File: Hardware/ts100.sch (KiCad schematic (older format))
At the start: 51 parts

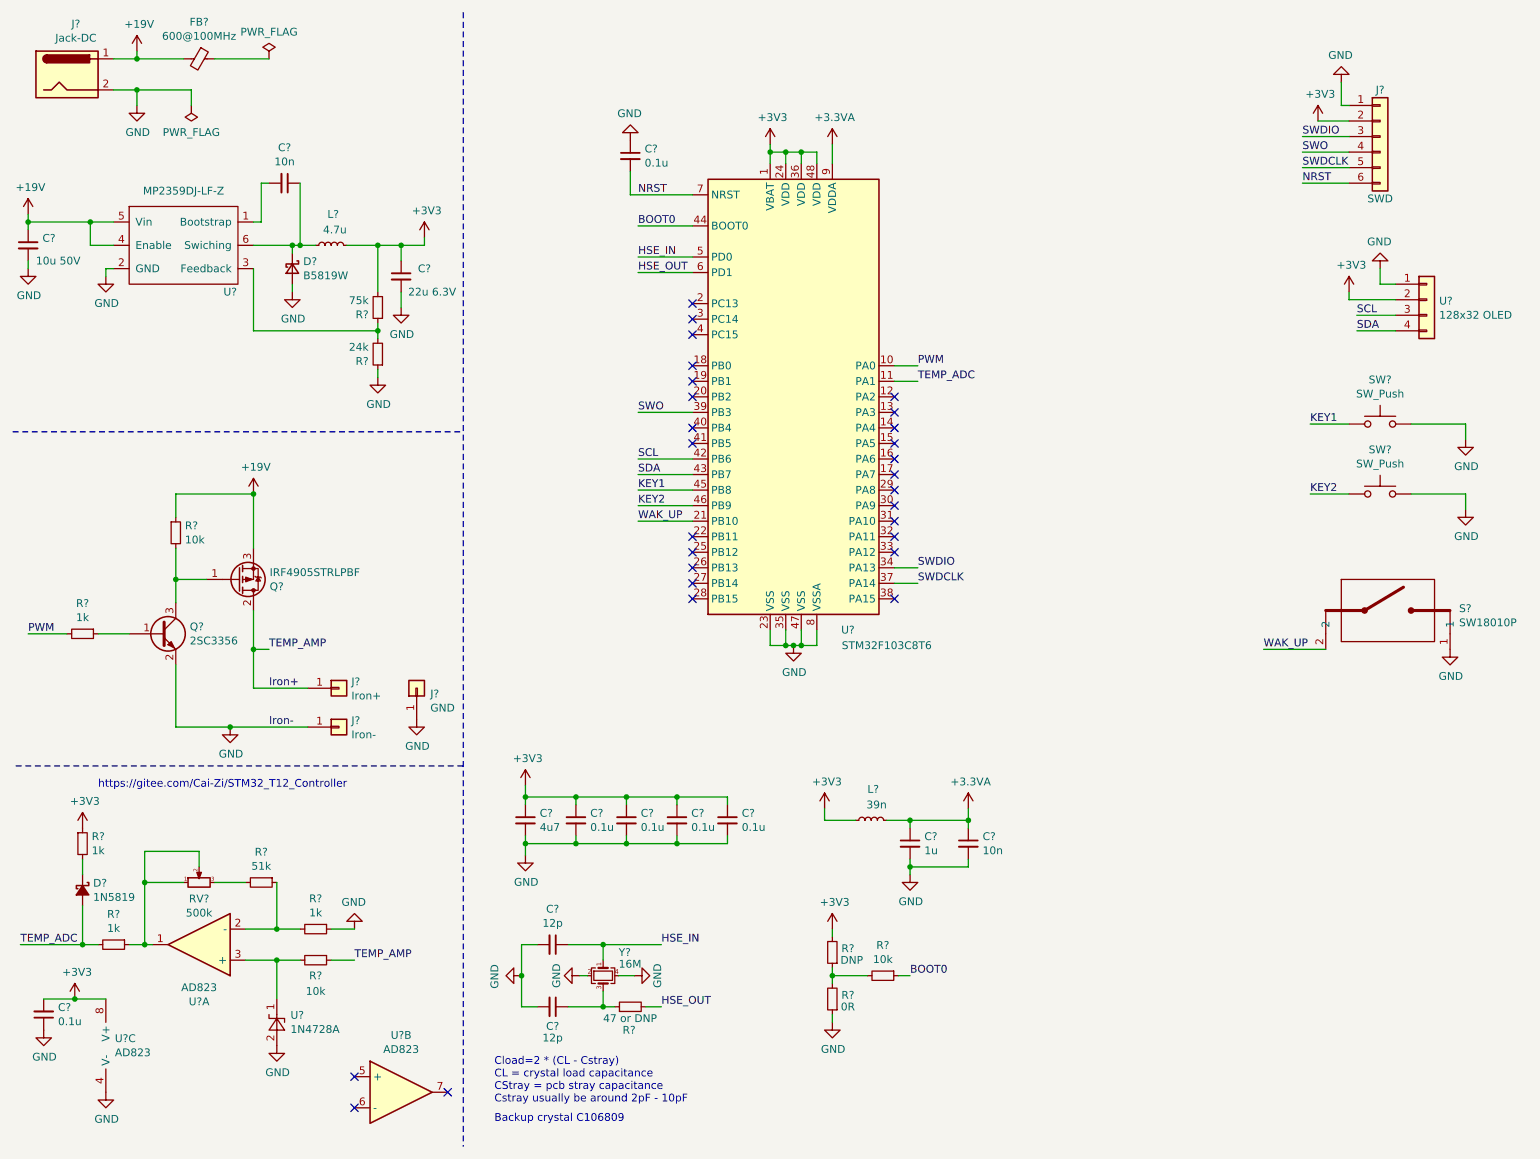
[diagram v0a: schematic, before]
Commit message: 修改封装
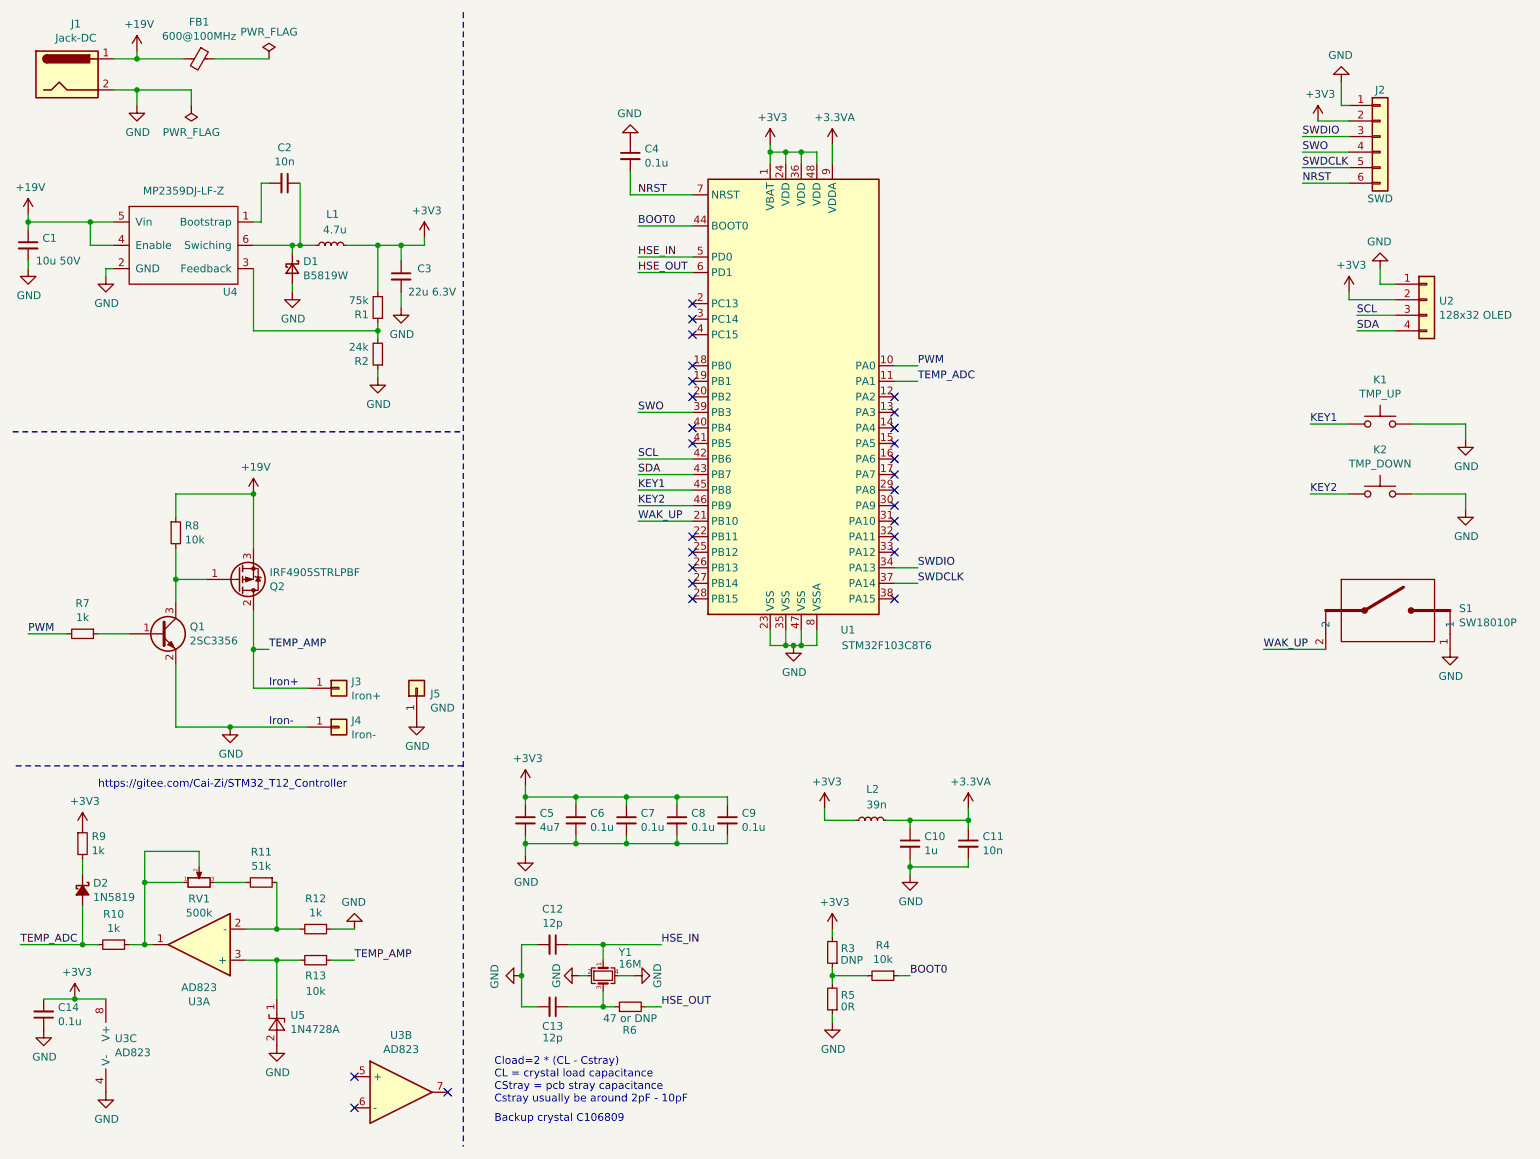
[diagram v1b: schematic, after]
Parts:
- D2: renamed from D?; footprint Diode_SMD:D_SMA -> Diode_SMD:D_SOD-123
- K1: renamed from SW?; value SW_Push -> TMP_UP
- K2: renamed from SW?; value SW_Push -> TMP_DOWN
- L1: renamed from L?; footprint ts100:Inductor_SMD_5x4.5mm -> Inductor_SMD:L_1008_2520Metric
- U5: renamed from U?; footprint Diode_THT:D_DO-41_SOD81_P7.62mm_Horizontal -> Diode_SMD:D_SOD-123
- gave numbers to parts that had none: 44

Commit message: 重绘PCB
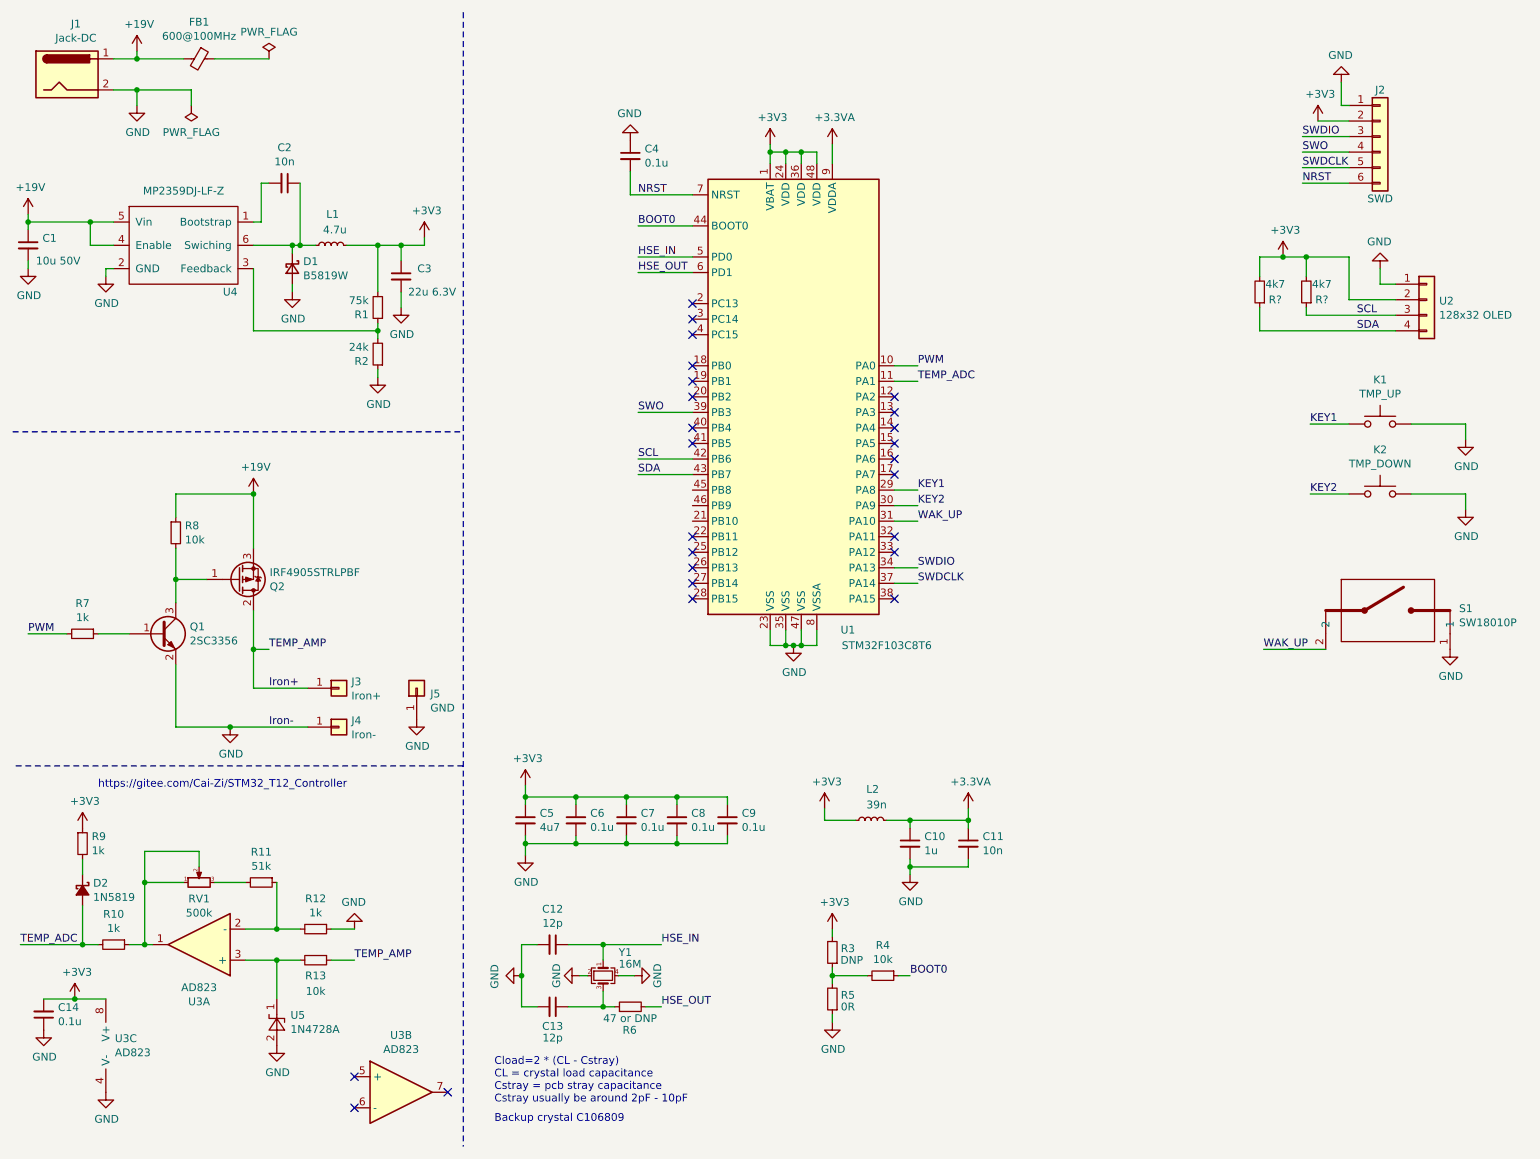
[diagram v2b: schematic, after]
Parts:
- added R? (x2): 4k7, Resistor_SMD:R_0402_1005Metric, symbol Device:R_Small
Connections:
- net +3V3: now also R?.2, R?.2
- net KEY1: now also U1.29 (PA8); no longer U1.45 (PB8)
- net KEY2: now also U1.30 (PA9); no longer U1.46 (PB9)
- net SCL: now also R?.1
- net SDA: now also R?.1
- net WAK_UP: now also U1.31 (PA10); no longer U1.21 (PB10)
- no-connect marks 28 -> 25
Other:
- note added: "Cload=2 * (CL - Cstray)\nCL = crystal load capacitance\nCstray = pcb stray capacitance\nCstray usually be around 2pF - 10pF"
- note removed: "Cload=2 * (CL - Cstray)\nCL = crystal load capacitance\nCStray = pcb stray capacitance\nCstray usually be around 2pF - 10pF"
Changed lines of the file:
@@
 encoding utf-8
 Sheet 1 1
-Title ""
-Date ""
+Title "Custom ts100 soldering iron"
+Date "2021-12-31"
 Rev ""
-Comp ""
-Comment1 ""
+Comp "liyuqihxc"
+Comment1 "https://github.com/liyuqihxc"
 Comment2 ""
 Comment3 ""
@@
 $EndComp
 $Comp
-L Reference_Voltage:LM4040DBZ-8.2 U5
-U 1 1 614593C0
-P 2200 7050
-F 0 "U5" V 2246 6962 50  0000 R CNN
-F 1 "1N4728A" V 2155 6962 50  0000 R CNN
-F 2 "Diode_SMD:D_SOD-123" H 2200 6850 50  0001 C CIN
-F 3 "http://www.ti.com/lit/ds/symlink/lm4040-n.pdf" H 2200 7050 50  0001 C CIN
-F 4 "C140852" H 2200 7050 50  0001 C CNN "PartNum"
-	1    2200 7050
-	0    -1   -1   0
-$EndComp
-$Comp
 L Device:R_POT_Small RV1
 U 1 1 6145A5F8
@@
 L power:+3V3 #PWR035
 U 1 1 615958C8
-P 9100 2350
-F 0 "#PWR035" H 9100 2200 50  0001 C CNN
-F 1 "+3V3" H 9115 2523 50  0000 C CNN
-F 2 "" H 9100 2350 50  0001 C CNN
-F 3 "" H 9100 2350 50  0001 C CNN
-	1    9100 2350
+P 8675 2125
+F 0 "#PWR035" H 8675 1975 50  0001 C CNN
+F 1 "+3V3" H 8690 2298 50  0000 C CNN
+F 2 "" H 8675 2125 50  0001 C CNN
+F 3 "" H 8675 2125 50  0001 C CNN
+	1    8675 2125
 	1    0    0    -1
 $EndComp
@@
 Wire Wire Line
 	9400 2400 9100 2400
-Wire Wire Line
-	9100 2400 9100 2350
 Text Label 9150 2500 0    50   ~ 0
 SCL
 Text Label 9150 2600 0    50   ~ 0
 SDA
-Wire Wire Line
-	9400 2500 9150 2500
-Wire Wire Line
-	9400 2600 9150 2600
 Wire Wire Line
 	1700 6050 1700 5950
@@
 NoConn ~ 6175 4025
 NoConn ~ 6175 3925
-NoConn ~ 6175 3825
-NoConn ~ 6175 3725
-NoConn ~ 6175 3625
 NoConn ~ 6175 3525
 NoConn ~ 6175 3425
@@
 Wire Wire Line
 	8950 4650 8550 4650
-Text Label 4525 3625 0    50   ~ 0
+Text Label 6325 3625 0    50   ~ 0
 KEY1
-Text Label 4525 3725 0    50   ~ 0
+Text Label 6325 3725 0    50   ~ 0
 KEY2
-Text Label 4525 3825 0    50   ~ 0
-WAK_UP
-Wire Wire Line
-	4875 3625 4525 3625
-Wire Wire Line
-	4525 3725 4875 3725
-Wire Wire Line
-	4875 3825 4525 3825
 Wire Wire Line
 	9050 1000 9050 1150
@@
 	4300 6950 4375 6950
 Text Notes 3600 7575 0    50   ~ 0
-Cload=2 * (CL - Cstray)\nCL = crystal load capacitance\nCStray = pcb stray capacitance\nCstray usually be around 2pF - 10pF
+Cload=2 * (CL - Cstray)\nCL = crystal load capacitance\nCstray = pcb stray capacitance\nCstray usually be around 2pF - 10pF
 $Comp
 L KIGIT_DC-DC:MP2359DJ-LF-Z U4
@@
 	600  1900 1000 1900
 Connection ~ 1000 1900
+$Comp
+L Reference_Voltage:LM4040DBZ-8.2 U5
+U 1 1 614593C0
+P 2200 7050
+F 0 "U5" V 2246 6962 50  0000 R CNN
+F 1 "1N4728A" V 2155 6962 50  0000 R CNN
+F 2 "Diode_SMD:D_SOD-123" H 2200 6850 50  0001 C CIN
+F 3 "http://www.ti.com/lit/ds/symlink/lm4040-n.pdf" H 2200 7050 50  0001 C CIN
+F 4 "C140852" H 2200 7050 50  0001 C CNN "PartNum"
+	1    2200 7050
+	0    -1   -1   0
+$EndComp
+Text Label 6325 3825 0    50   ~ 0
+WAK_UP
+Wire Wire Line
+	6175 3625 6325 3625
+Wire Wire Line
+	6175 3725 6325 3725
+Wire Wire Line
+	6175 3825 6325 3825
+$Comp
+L Device:R_Small R?
+U 1 1 62117427
+P 8825 2350
+F 0 "R?" H 8725 2400 50  0000 C CNN
+F 1 "4k7" H 8725 2300 50  0000 C CNN
+F 2 "Resistor_SMD:R_0402_1005Metric" H 8825 2350 50  0001 C CNN
+F 3 "~" H 8825 2350 50  0001 C CNN
+	1    8825 2350
+	-1   0    0    1
+$EndComp
+$Comp
+L Device:R_Small R?
+U 1 1 62118B2E
+P 8525 2350
+F 0 "R?" H 8425 2400 50  0000 C CNN
+F 1 "4k7" H 8425 2300 50  0000 C CNN
+F 2 "Resistor_SMD:R_0402_1005Metric" H 8525 2350 50  0001 C CNN
+F 3 "~" H 8525 2350 50  0001 C CNN
+	1    8525 2350
+	-1   0    0    1
+$EndComp
+Wire Wire Line
+	8825 2125 8675 2125
+Wire Wire Line
+	8525 2125 8525 2250
+Wire Wire Line
+	8825 2125 8825 2250
+Connection ~ 8675 2125
+Wire Wire Line
+	8675 2125 8525 2125
+Wire Wire Line
+	8825 2125 9100 2125
+Wire Wire Line
+	9100 2125 9100 2400
+Connection ~ 8825 2125
+Wire Wire Line
+	8825 2450 8825 2500
+Wire Wire Line
+	8825 2500 9400 2500
+Wire Wire Line
+	8525 2450 8525 2600
+Wire Wire Line
+	8525 2600 9400 2600
 $EndSCHEMATC
